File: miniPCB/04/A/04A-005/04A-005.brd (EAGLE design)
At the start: 24 parts

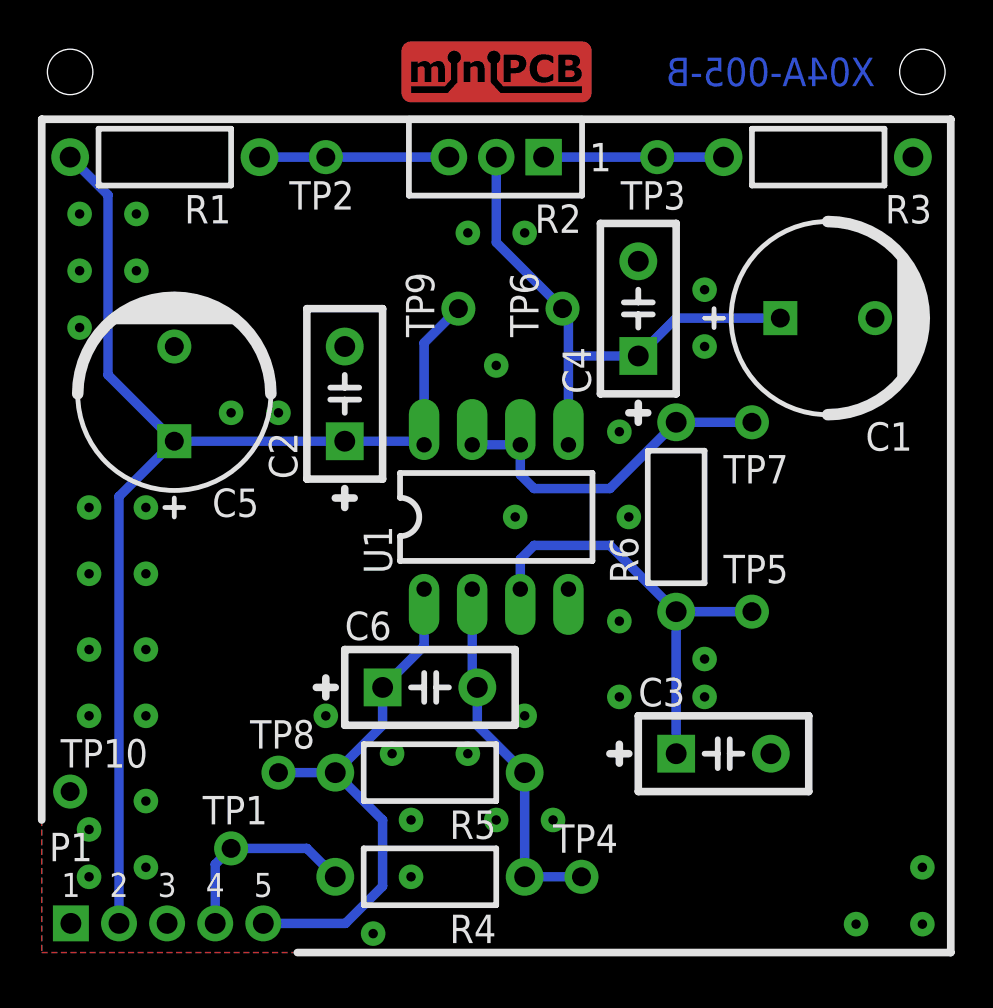
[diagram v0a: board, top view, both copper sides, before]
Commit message: NM.03SEP2023
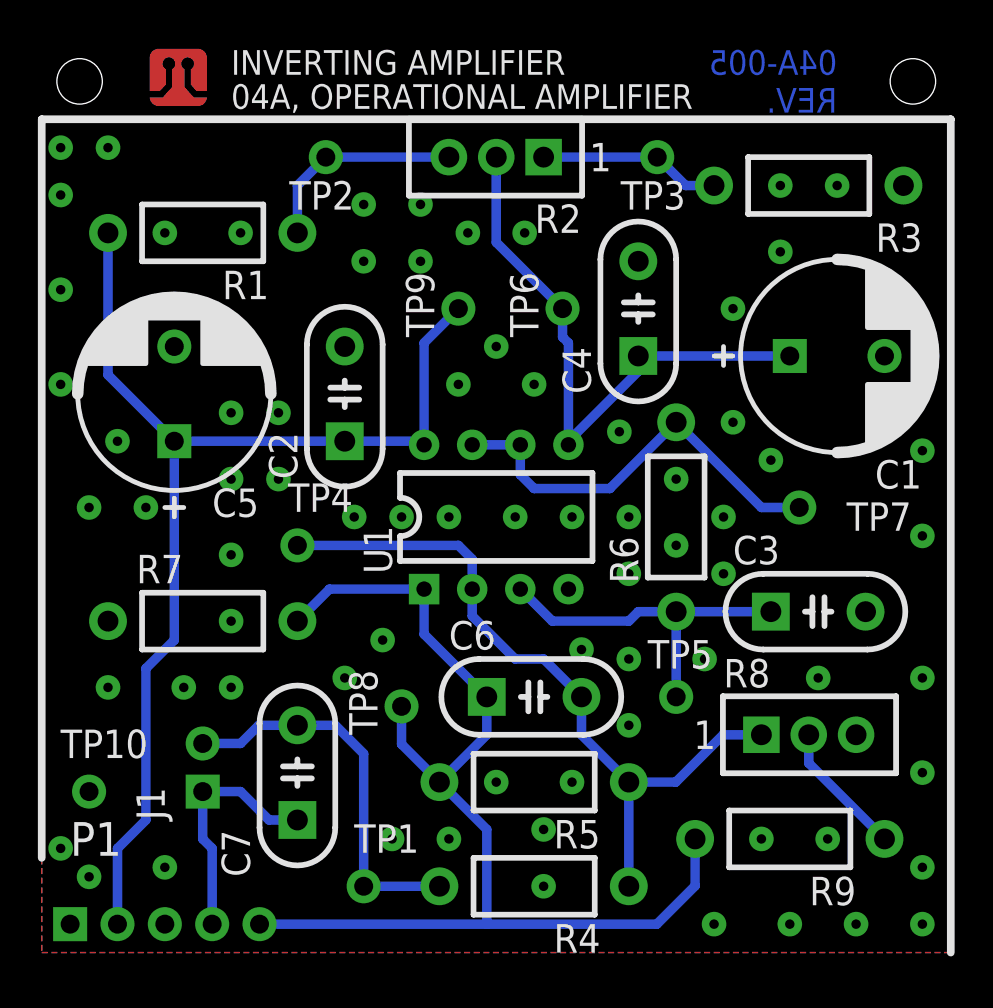
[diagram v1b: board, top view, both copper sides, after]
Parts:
- removed P1-: (no value), minipcb:MINIPCB_5P_50X50MM
- added C7: (no value), minipcb:C050-024X044
- added J1: JUMPER, minipcb:PINS_2
- added P1: (no value), minipcb:PINS_1X5
- added R7, R9: (no value), minipcb:0207/10
- added R8: (no value), minipcb:TRIM_0100
- added U$1: MINIPCB_50X50, minipcb:MINIPCB_0P_50X50MM
- moved TP4 23.0 mm to (14.5, 22.5)
- moved C3 9.01 mm to (42.0, 19.0)
- moved TP8 7.38 mm to (20.0, 14.0), turned to 90 degrees
- moved TP1 7.28 mm to (18.0, 4.50)
- moved TP5 6.02 mm to (34.5, 14.5)
- moved C6 5.52 mm to (27.0, 14.5)
- moved R4 5.52 mm to (27.0, 4.50)
- moved R5 5.52 mm to (27.0, 10.0)
- moved TP7 5.15 mm to (41.0, 24.5)
- moved R1 4.47 mm to (9.50, 39.0)
- moved C1 2.06 mm to (43.0, 32.5)
- moved R3 1.58 mm to (41.5, 41.5)
- moved TP10 1.00 mm to (3.50, 9.50)
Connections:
- net N$1 renamed VR
- net N$3 renamed VREF+
- new net IN-DC: C7.2, J1.2, R4.2, TP1.1
- new net N$1: R8.2, R9.1
- net GND: now also P1.1, R7.1; no longer P1-.1
- net IN: now also C7.1, J1.1, P1.4; no longer P1-.4, R4.2, TP1.1
- net NC: now also P1.3; no longer P1-.3
- net OUT: now also P1.5, R7.2, R9.2; no longer P1-.5
- net V+: now also P1.2; no longer P1-.2
- net VFB: now also R8.1
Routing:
- net OUT: track 28.8 -> 59.7 mm
- net IN-DC: track 0.00 -> 20.5 mm
- net VFB: track 19.3 -> 39.1 mm
- net N$1: track 0.00 -> 7.16 mm
- net V+: track 65.2 -> 60.4 mm
- net VREF+: track 23.1 -> 18.6 mm
- net VREF: track 18.1 -> 22.5 mm
- net IN: track 10.4 -> 12.8 mm
- net VR: track 28.8 -> 30.8 mm
- net P1.3: track 10.0 -> 11.1 mm
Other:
- board text added: "C7"
- board text added: "J1"
- board text added: "R7"
- board text added: "R8"
- board text added: "R9"
- board text removed: "INVERTING AMPLIFIER"
